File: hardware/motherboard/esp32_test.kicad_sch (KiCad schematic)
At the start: 17 parts, among them J2 USB C 2.0, Q1 TSM7P06CP_ROG, U1 ESP32-S3-WROOM-1, U2 TPS75533KTTRG3

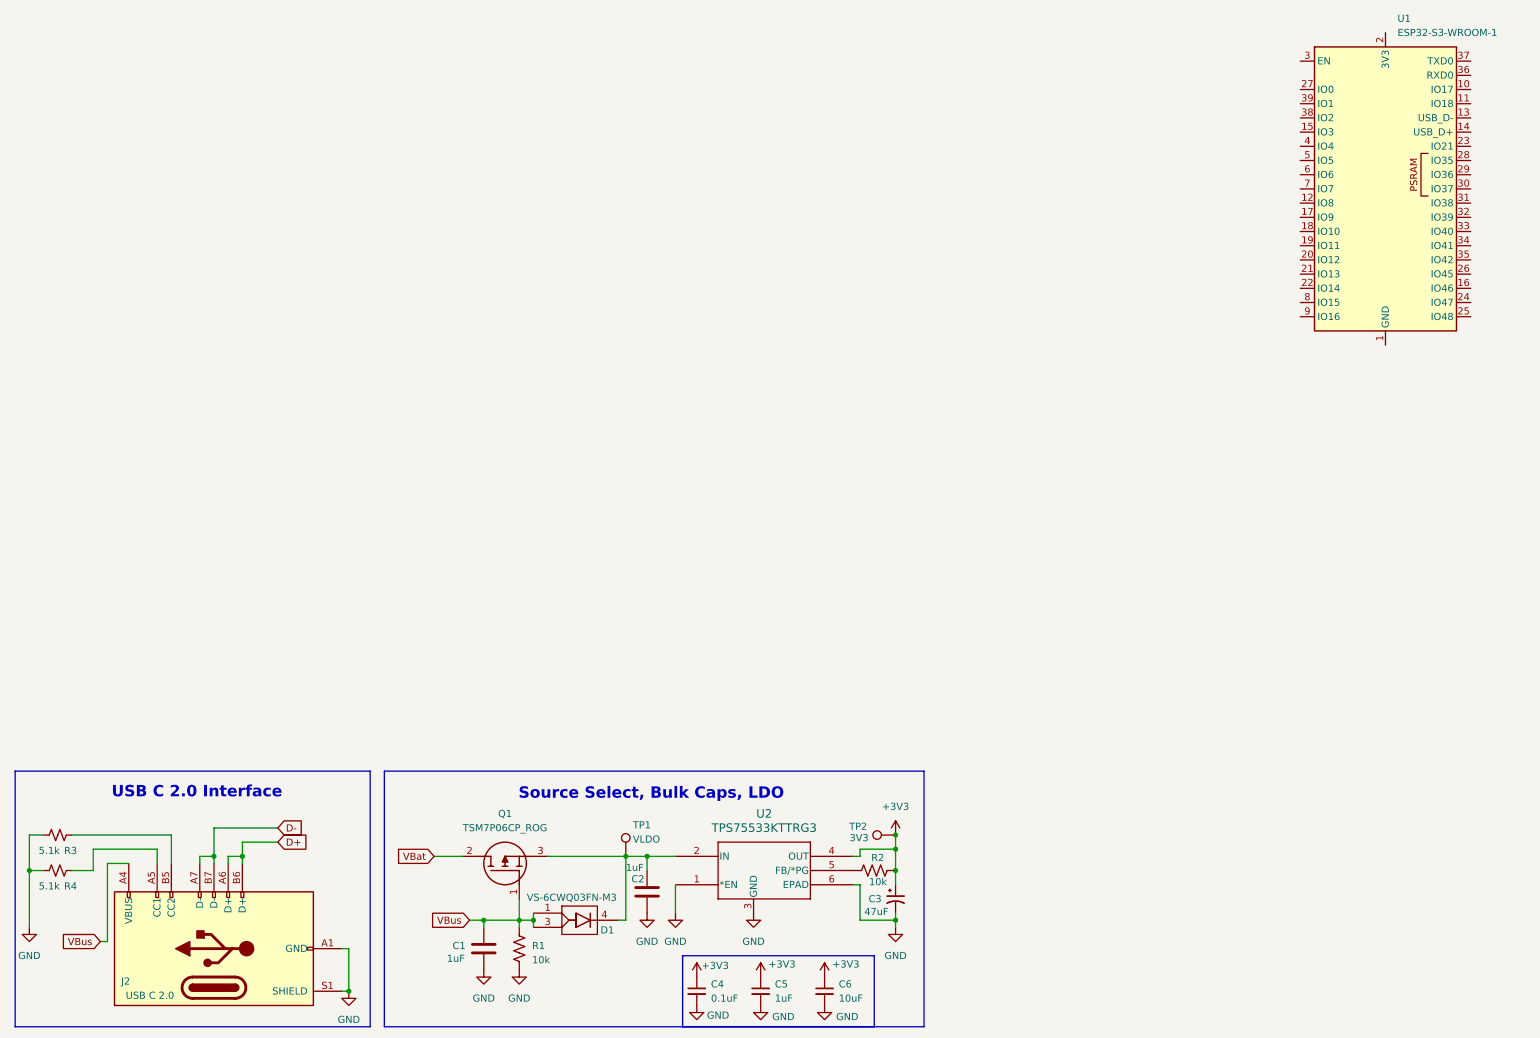
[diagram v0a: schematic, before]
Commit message: Basic Microcontroller Stuff and Display Power
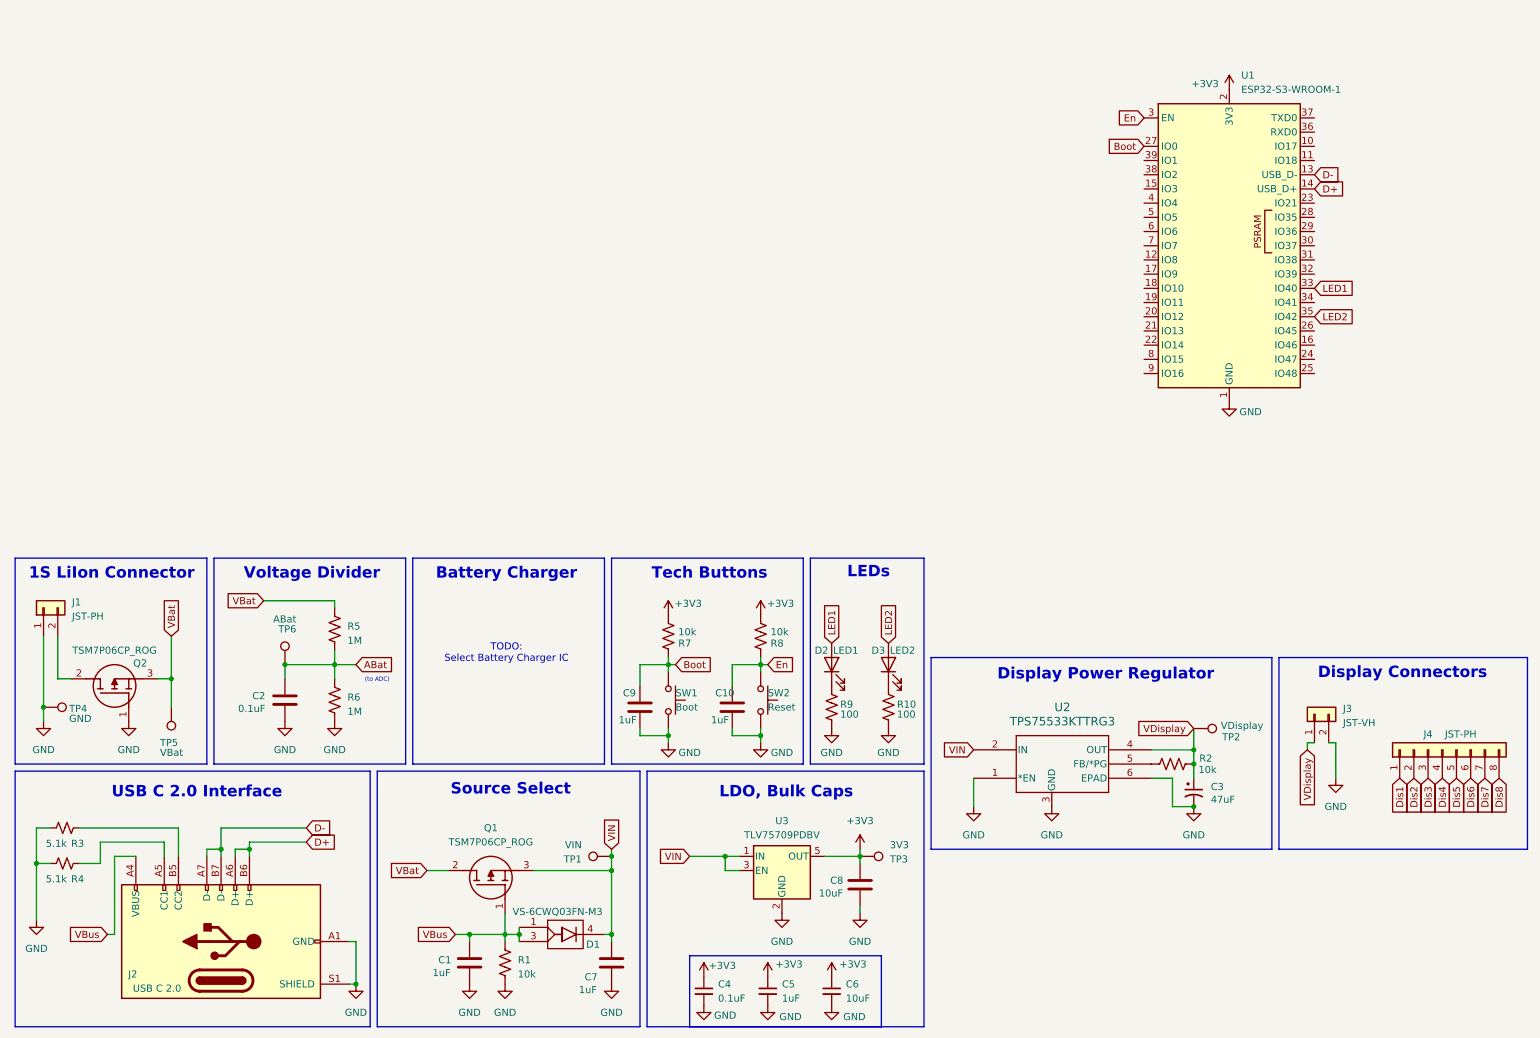
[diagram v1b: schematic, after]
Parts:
- added C10, C7, C9: 1uF, symbol Device:C
- added C8: 10uF, symbol Device:C
- added D2: LED1, symbol Device:LED
- added D3: LED2, symbol Device:LED
- added J1: JST-PH, symbol Connector_Generic:Conn_01x02
- added J3: JST-VH, symbol Connector_Generic:Conn_01x02
- added J4: JST-PH, symbol Connector_Generic:Conn_01x08
- added Q2: TSM7P06CP_ROG, TSM7P06CPROG, symbol Library_Loader:TSM7P06CP_ROG
- added R10, R9: 100, symbol Device:R_US
- added R5, R6: 1M, symbol Device:R_US
- added R7, R8: 10k, symbol Device:R_US
- added SW1: Boot, symbol Switch:SW_Push
- added SW2: Reset, symbol Switch:SW_Push
- added TP3: 3V3, symbol Connector:TestPoint
- added TP4: GND, symbol Connector:TestPoint
- added TP5: VBat, symbol Connector:TestPoint
- added TP6: ABat, symbol Connector:TestPoint
- added U3: TLV75709PDBV, Package_TO_SOT_SMD:SOT-23-5, symbol Regulator_Linear:TLV75709PDBV
- C2: value 1uF -> 0.1uF
- TP1: value VLDO -> VIN
- TP2: value 3V3 -> VDisplay
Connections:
- net +3V3: now also U1.2 (3V3), C8.1, R7.2, R8.2, TP3.1, U3.5 (OUT); no longer C3.1, R2.2, TP2.1, U2.4 (OUT)
- net D+: now also U1.14 (USB_D+)
- net D-: now also U1.13 (USB_D-)
- net GND: now also U1.1 (GND), U1.40 (GND), U1.41 (GND), C10.2, C7.2, C8.2, C9.2, J1.1 (Pin_1), J3.2 (Pin_2), Q2.1 (G), R10.1, R6.2, R9.1, SW1.2, SW2.2, TP4.1, U3.2 (GND)
- net VBat: now also Q2.3 (S), R5.1, TP5.1
- net VIN: now reaches D1.4, Q1.3 (S), TP1.1, U2.2 (IN)
- net VIN: now also C7.1, U3.1 (IN), U3.3 (EN); no longer C2.1
- net Boot: now reaches U1.27 (IO0)
- net Boot: now also C9.1, R7.1, SW1.1
- net En: now reaches U1.3 (EN)
- net En: now also C10.1, R8.1, SW2.1
- net LED1: now reaches U1.33 (IO40)
- net LED1: now also D2.2 (A)
- net LED2: now reaches U1.35 (IO42)
- net LED2: now also D3.2 (A)
- new net: J1.2 (Pin_2), Q2.2 (D)
- new net: D2.1 (K), R9.2
- new net: D3.1 (K), R10.2
- new net ABat: C2.1, R5.2, R6.1, TP6.1
- new net Dis1: J4.1 (Pin_1)
- new net Dis2: J4.2 (Pin_2)
- new net Dis3: J4.3 (Pin_3)
- new net Dis4: J4.4 (Pin_4)
- new net Dis5: J4.5 (Pin_5)
- new net Dis6: J4.6 (Pin_6)
- new net Dis7: J4.7 (Pin_7)
- new net Dis8: J4.8 (Pin_8)
- new net VDisplay: C3.1, J3.1 (Pin_1), R2.2, TP2.1, U2.4 (OUT)
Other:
- note added: "(to ADC)"
- note added: "1S LiIon Connector"
- note added: "Battery Charger"
- note added: "Display Connectors"
- note added: "Display Power Regulator"
- note added: "LDO, Bulk Caps"
- note added: "LEDs"
- note added: "Source Select"
- note added: "TODO: Select Battery Charger IC"
- note added: "Tech Buttons"
- note added: "Voltage Divider"
- note removed: "Source Select, Bulk Caps, LDO"
- company: (none) -> "Gamers"
- title: (none) -> Handheld Game Motherboard
- moved on the sheet: C1, C3, C4, C5, C6, D1, J2, Q1, R1, R2, R3, R4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
